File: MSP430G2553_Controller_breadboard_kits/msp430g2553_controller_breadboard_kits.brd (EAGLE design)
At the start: 16.7 x 39.5 mm, 12 parts, among them J3 programmer header, U1 MSP430G2553_24IO_28PIN_TSSOP

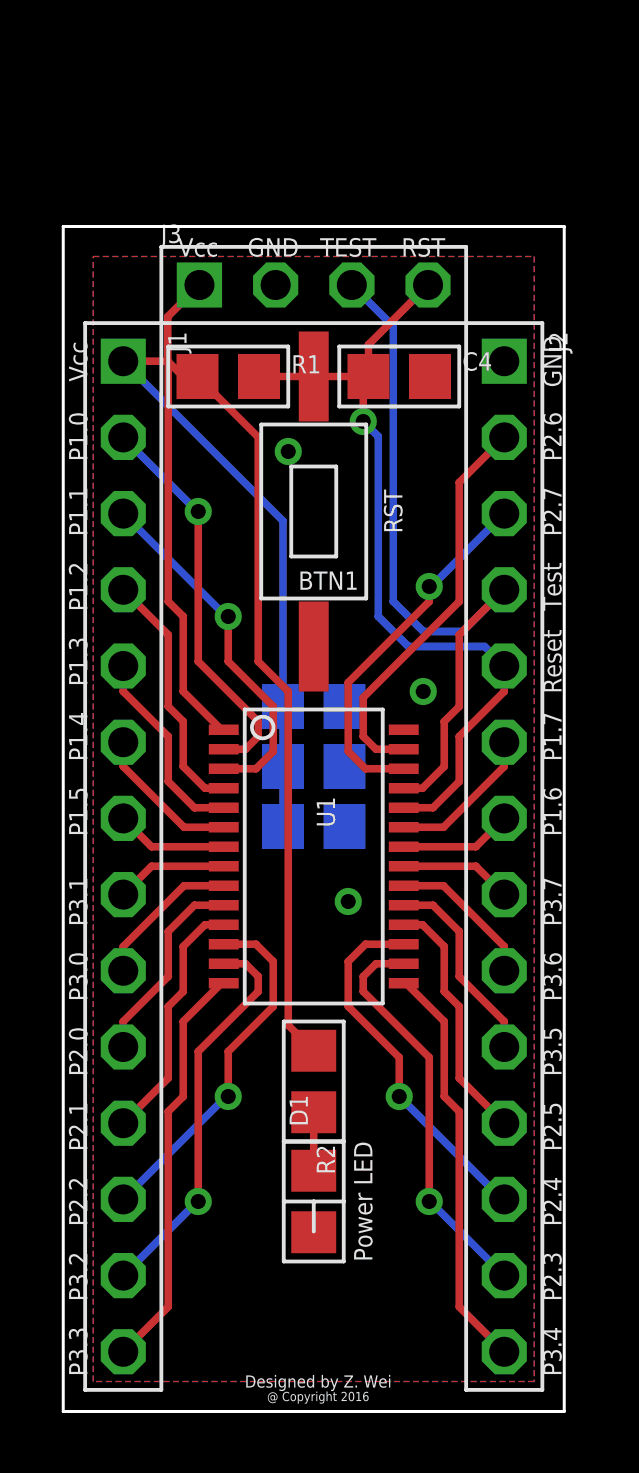
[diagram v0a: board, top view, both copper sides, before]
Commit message: done the design
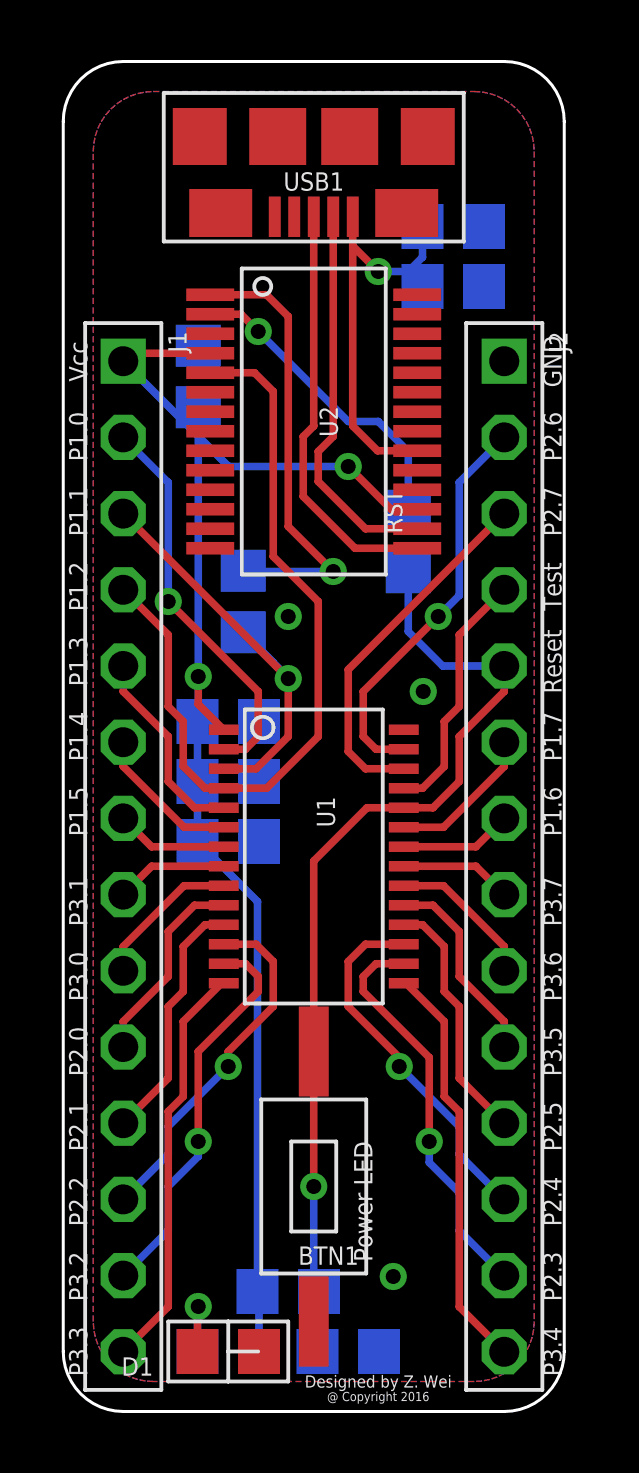
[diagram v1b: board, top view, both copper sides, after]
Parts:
- removed J3: programmer header, Connectors:4PIN_HEADER_PITCH2.54MM_TH
- added C5: 0.1uF, Capacitors:0805
- added C6, C7, C8: (no value), Capacitors:0805
- added R5: (no value), Resistors:0805
- added U2: (no value), FTDI:SSOP-28
- added USB1: (no value), Connectors:MICRO-USB-B-SMD-SMD
- moved C4 32.5 mm to (9.50, 2.00), flipped to the bottom, turned to 180 degrees
- moved R1 30.6 mm to (7.50, 4.00), flipped to the bottom, turned to 180 degrees
- moved BTN1 22.5 mm to (8.35, 7.50)
- moved R2 9.44 mm to (5.50, 2.00), flipped to the bottom, turned to 0 degrees
- moved D1 5.76 mm to (5.50, 2.00), turned to 180 degrees
- moved C1 2.89 mm to (5.50, 19.0)
- moved C2 2.89 mm to (5.50, 21.0)
- moved C3 2.89 mm to (5.50, 23.0)
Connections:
- removed net P1.1: J1.3, U1.3
- removed net P1.2: J1.4, U1.4
- new net +5V: C7.1, C8.1, U2.20, USB1.1
- new net DTR: C5.2, U2.2
- new net RX: J1.3, R5.2, U1.3
- new net TX: J1.4, U1.4, U2.5
- new net TXO: R5.1, U2.1
- new net USBDM: U2.16, USB1.2
- new net USBDP: U2.15, USB1.3
- net +3V3: now also C6.1, U2.17, U2.4; no longer J3.1
- net DGND: now also C6.2, C7.2, C8.2, U2.18, U2.21, U2.25, U2.26, U2.7, USB1.5, USB1.S1, USB1.S2; no longer J3.2
- net RST: now also C5.1; no longer J3.4
- net TEST: no longer J3.3
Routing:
- net TX: track 0.00 -> 26.7 mm
- net TEST: track 24.2 -> 8.37 mm
- net TXO: track 0.00 -> 15.0 mm, vias 0 -> 1
- net RX: track 0.00 -> 14.5 mm, vias 0 -> 1
- net +5V: track 0.00 -> 14.1 mm, vias 0 -> 1
- net USBDP: track 0.00 -> 14.0 mm
- net USBDM: track 0.00 -> 13.0 mm
- net +3V3: track 61.8 -> 49.3 mm, vias 0 -> 2
- net P1.1: track 11.9 -> 0.00 mm, vias 1 -> 0
- net DTR: track 0.00 -> 10.5 mm, vias 0 -> 1
- net P1.2: track 8.37 -> 0.00 mm
- net RST: track 27.4 -> 32.5 mm
- net N$2: track 1.95 -> 3.02 mm, vias 0 -> 1
- net P2.7: vias 1 -> 0
- net P2.6: vias 0 -> 1
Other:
- board size 16.7 x 39.5 mm -> 16.7 x 45 mm
- board text removed: "TEST"
